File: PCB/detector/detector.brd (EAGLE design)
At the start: 53.3 x 51.7 mm, 36 parts, among them IC1 STM32F042K6T6

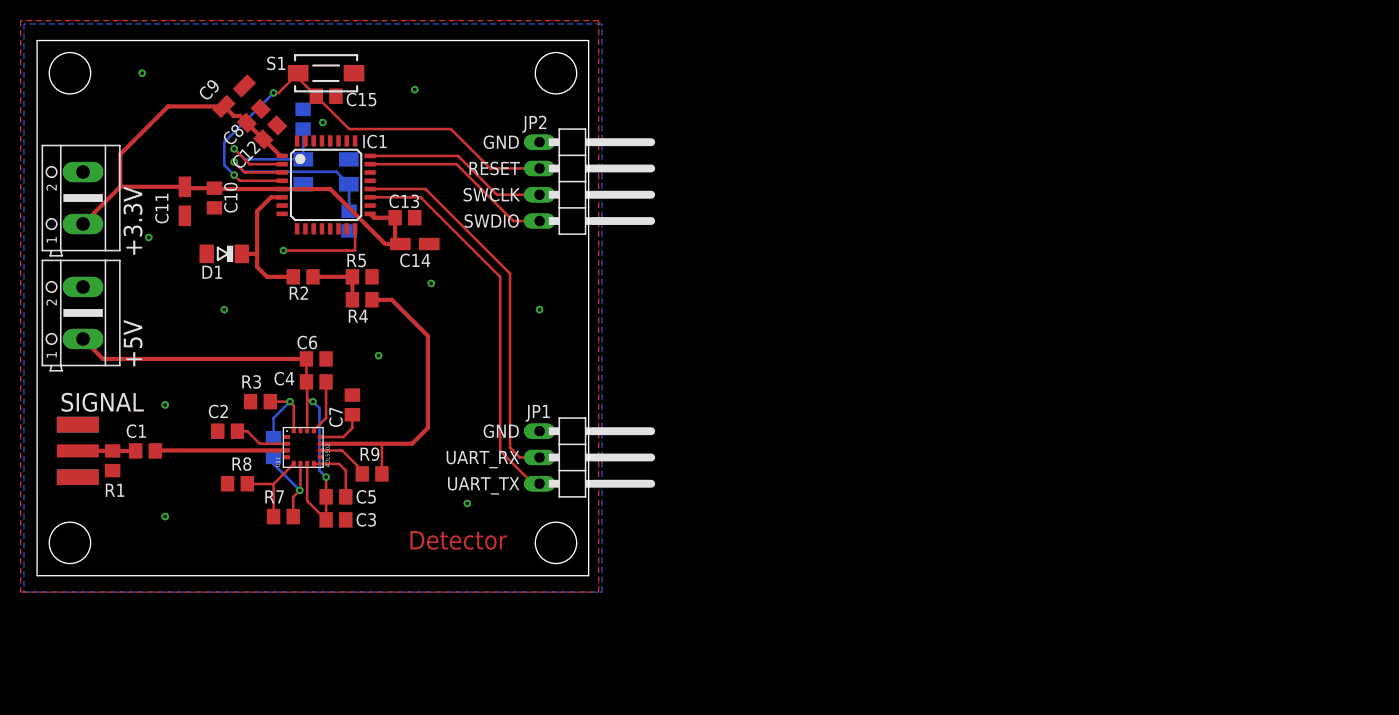
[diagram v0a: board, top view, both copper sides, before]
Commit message: almost ready
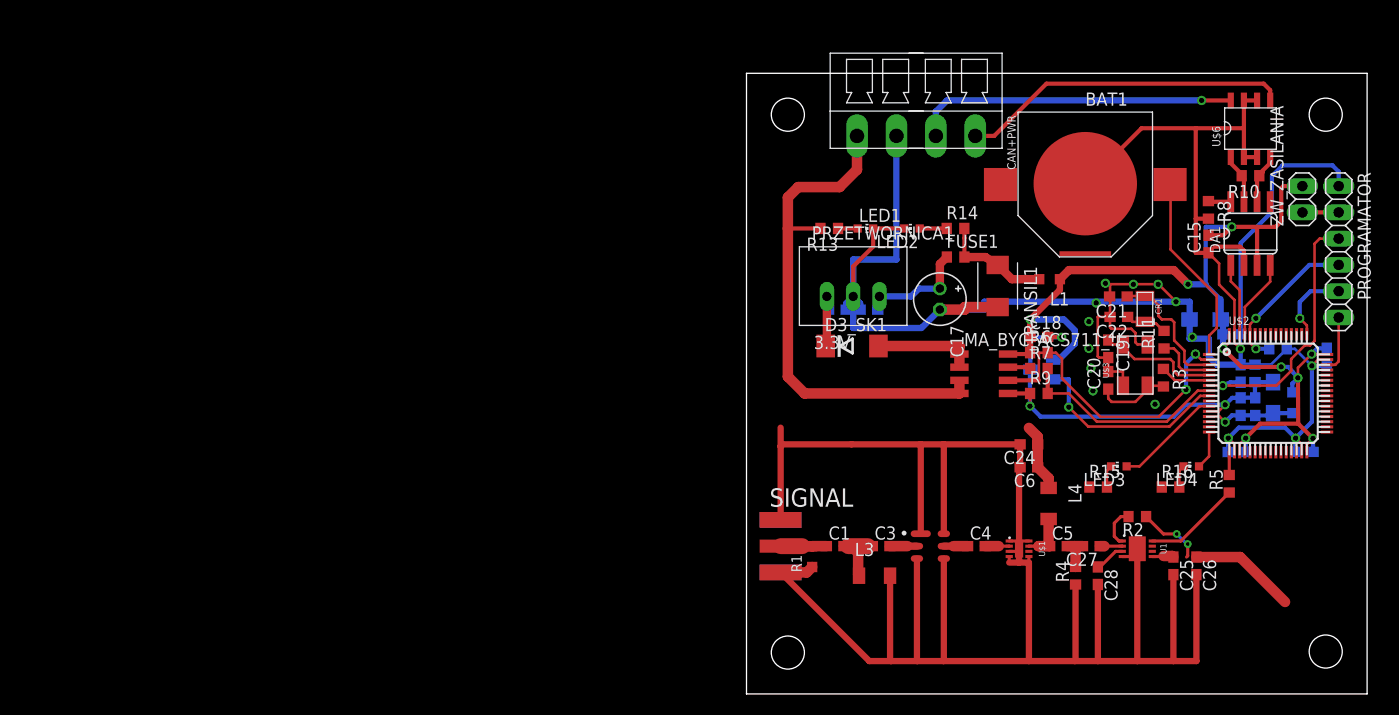
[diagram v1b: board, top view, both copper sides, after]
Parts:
- removed +3.3V, +5V: (no value), con-ptr500:AK500/2
- removed D1: 3.3V, diode:SOD80C
- removed JP1: (no value), pinhead:1X03/90
- removed JP2: (no value), pinhead:1X04/90
- removed Q1: (no value), crystal:CTS406
- removed S1: DTSM-3, swtich:DTSM-3
- added BAT1: BAT_3V, battery CR1216:CR1216
- added C18, C23: 100nF, resistor:C0603
- added C19, C20, C21, C22: 22pF, resistor:C0603
- added C24: 1u, rcl:C0603
- added C25: 100p, rcl:C0603
- added C26: 100n, rcl:C0603
- added C27, C28: 1n, rcl:C0603
- added CAN+PWR: 4PIN_3.81_KATOWA, zielone raster 3.81:CON-PHOENIX_3.81-4PIN_KAT
- added CR1: 32,768kHz, crystal_scorpio:IL3X
- added D3_SK1: 5A, diode:DO214AA
- added DA1: SN65HVD230, can_driver:SO08
- added FUSE1: 3A, resistor:R0603
- added L1: 1uH/500mA, rcl:L2012C
- added L2: 10uH/20mA, rcl:L2012C
- added L3, L4: (no value), rcl:L3216C
- added LED1, LED3: zielona, led:CHIP-LED0603
- added LED2: niebieska, led:CHIP-LED0603
- added LED4: czerwona, led:CHIP-LED0603
- added MA_BYC_ACS711_!!: ACS712, acs712:SO08
- added PROGRAMATOR: (no value), pinhead:1X06
- added PRZETWORNICA1: 3.3V, OKI-78SR:TO220
- added R10: 120R*, resistor:R0603
- added R11: 390k, resistor:R0603
- added R12, R13: 10k, resistor:R0603
- added R14, R15, R16: 470R, resistor:R0603
- added TRANSIL1: 3.3V, diode:SMBJ
- added U$2: STM32F072RBT6, STM32F072RBT6:TQFP64
- added U$3: ABM3, crystal_scorpio:ABM3
- added U$6: LC03-6R2G, LC03-6R2 - diody ESD do magistrali:SOIC-8
- added U1: LT5538, DFN-8:DFN-8_3X3
- added U2: B39431B3710U410, SON120P300X300X110-6N:SON120P300X300X110-6N
- added ZW_MASY: (no value), resistor:R0603
- added ZW_ZASILANIA: (no value), pinhead:1X02
- C1: value 100n -> (none); device rcl:C0805 -> rcl:C0603
- C10, C12, C15: value 100n -> 100nF; device rcl:C0805 -> resistor:C0603
- C11, C9: value 4.7u -> 100nF; device rcl:CT3216 -> resistor:C0603
- C13: value 10n -> 100nF; device rcl:C0805 -> resistor:C0603
- C14: value 1u -> 100nF; device rcl:CT3216 -> resistor:C0603
- C16: value 20p -> 100nF; device rcl:C0805 -> resistor:C0603
- C17: value 20p -> 6,3V/100uF; device rcl:C0805 -> resistor:E2-5
- C2: value 100p -> 4,7uF; device rcl:C0805 -> rcl:SMC_A
- C3: value 100p -> (none); device rcl:C0805 -> rcl:C0603
- C4: device rcl:C0805 -> rcl:C0603
- C5, C6: value 100n -> 100p; device rcl:C0805 -> rcl:C0603
- C7: value 10u -> 4,7uF; device rcl:C0805 -> rcl:SMC_A
- C8: value 100n -> 1uF; device rcl:C0805 -> resistor:C0603
- IC1: value STM32F042K6T6 -> LM50; device STM32F042K6T6:QFP80P900X900X160-32N -> linear:SOT23
- R1: value 60.4R -> VARISTORCN0603; device rcl:R0805 -> varistor:CT/CN0603
- R2: value 2k -> (none); device rcl:R0805 -> rcl:R0603
- R3: value 301R -> 820R; device rcl:R0805 -> resistor:R0603
- R4: value 10k -> 56R; device rcl:R0805 -> rcl:R0603
- R5: value 20k -> (none); device rcl:R0805 -> rcl:R0603
- R6: value 1430R -> 10k; device rcl:R0805 -> resistor:R0603
- R7: value 3.74k -> 100K; device rcl:R0805 -> resistor:R0603
- R8: value 2k -> ZW 0-100K; device rcl:R0805 -> resistor:R0603
- R9: value 0R -> 32k; device rcl:R0805 -> resistor:R0603
- U$1: value ADL5902 -> TQP3M9036; device ADL5902:ADL5902 -> DFN-8:DFN-8_2X2
- moved C11 111.4 mm to (127.2, 23.7), flipped to the bottom
- moved C9 101.8 mm to (118.9, 18.9), flipped to the bottom, turned to 90 degrees
- moved C8 100.8 mm to (120.3, 18.9), flipped to the bottom, turned to 90 degrees
- moved C10 99.2 mm to (118.0, 25.9), flipped to the bottom, turned to 180 degrees
- moved C12 98.4 mm to (118.5, 14.5), flipped to the bottom, turned to 0 degrees
- moved R8 97.5 mm to (115.8, 37.9), turned to 270 degrees
- moved C2 95.1 mm to (115.5, 27.3), flipped to the bottom, turned to 0 degrees
- moved C13 89.8 mm to (125.0, 14.5), flipped to the bottom
- moved C7 89.0 mm to (122.0, 19.8), flipped to the bottom
- moved R3 87.3 mm to (111.4, 21.7), turned to 270 degrees
- moved C15 86.5 mm to (115.8, 34.6), turned to 90 degrees
- moved R5 86.2 mm to (117.8, 11.4), turned to 90 degrees
- moved R2 83.9 mm to (108.9, 8.26), turned to 180 degrees
- moved R6 74.6 mm to (99.4, 24.1), flipped to the top, turned to 0 degrees
- moved R7 74.4 mm to (99.4, 22.6)
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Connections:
- net N$1 renamed SIGNAL
- removed net +5V: +5V.1, C3.1, C4.1, C5.1, C6.1, U$1.P$10, U$1.P$3
- removed net ADC_IN: D1.C, IC1.6, R2.1
- removed net INHI: C1.2, U$1.P$14
- removed net OSC_IN: C17.1, IC1.2, Q1.3
- removed net OSC_OUT: C16.1, IC1.3, Q1.1
- removed net RESET: C15.1, IC1.4, JP2.2, S1.1
- removed net SWCLK: IC1.24, JP2.3
- removed net UART_RX: IC1.20, JP1.2
- removed net UART_TX: IC1.19, JP1.3
- removed net VOUT: R4.2, R9.2, U$1.P$6
- new net +24V: C14.1, D3_SK1.C, PRZETWORNICA1.P1
- new net AGND: C18.2, C7.-, C8.2, C9.2, IC1.3, MA_BYC_ACS711_!!.5, R9.1, U$2.12, ZW_MASY.2
- new net AMP_OUT: C27.2, C5.2, R4.2
- new net BOOT_0: PROGRAMATOR.4, R12.2, U$2.60
- new net CANH_1: DA1.7, R10.2, U$6.1
- new net CANL_1: DA1.6, R10.1, U$6.4
- new net CAN_RX_1: DA1.4, U$2.61
- new net CAN_TX_1: DA1.1, U$2.62
- new net DET_OUT: R5.2, U$2.17
- new net FILTER_IN: C3.2, U2.2
- new net FILTER_OUT: C4.1, U2.5
- new net LED1: LED3.A, U$2.11
- new net LED2: LED4.A, U$2.16
- new net N$1: MA_BYC_ACS711_!!.7, R7.1
- new net N$10: C19.1, U$2.5, U$3.P$2
- new net N$11: C4.2, U$1.2
- new net N$12: CAN+PWR.P$2, U$6.8
- new net N$13: R11.1, U$2.4
- new net N$14: C21.1, CR1.P$1, U$2.3
- new net N$15: C22.1, CR1.P$2, R11.2
- new net N$16: CAN+PWR.P$1, U$6.5
- new net N$18: LED1.A, R13.1
- new net N$19: LED2.A, R14.1
- new net N$20: LED3.C, R15.2
- new net N$21: LED4.C, R16.2
- new net N$22: C28.1, U1.3
- new net N$23: C27.1, U1.2
- new net N$24: PROGRAMATOR.2, ZW_ZASILANIA.1
- new net N$25: R2.2, U1.1
- new net N$27: C5.1, L4.2, U$1.7
- new net N$28: U1.7
- new net N$29: U1.6
- new net N$8: D3_SK1.A, MA_BYC_ACS711_!!.1, MA_BYC_ACS711_!!.2
- new net NRST: C23.1, PROGRAMATOR.3, U$2.7
- new net OVER_CURRENT: MA_BYC_ACS711_!!.6, R6.2, U$2.2
- new net PRAD_PLYTKI: R7.2, R9.2, U$2.8
- new net SWD_CLK: PROGRAMATOR.5, U$2.49
- new net TEMP: IC1.2, U$2.9
- new net VBAT: BAT1.P$1, BAT1.P$2, BAT1.P$3, U$2.1
- new net VCC: CAN+PWR.P$4, MA_BYC_ACS711_!!.3, MA_BYC_ACS711_!!.4, R13.2
- new net VDD: C10.1, C11.1, C12.1, C13.1, C15.2, C18.1, C2.+, DA1.3, IC1.1, L1.1, L2.1, MA_BYC_ACS711_!!.8, R6.1, U$2.19, U$2.32, U$2.48, U$2.64, ZW_ZASILANIA.2
- net +3V3: now also C24.1, C25.1, C26.1, C6.1, FUSE1.2, L1.2, L4.1, R14.2, R2.1, TRANSIL1.C, U1.5; no longer +3.3V.1, C10.1, C11.+, C12.1, C13.1, C14.+, C8.1, C9.+, IC1.1, IC1.17, IC1.5
- net GND: now also BAT1.P$4, C11.2, C14.2, C15.1, C17.-, C19.2, C2.-, C20.2, C21.2, C22.2, C23.2, C24.2, C25.2, C26.2, C28.2, CAN+PWR.P$3, DA1.2, L3.2, LED1.C, LED2.C, PROGRAMATOR.1, PRZETWORNICA1.P2, R12.1, R15.1, R16.1, R4.1, R8.2, TRANSIL1.A, U$1.1, U$1.3, U$1.4, U$1.5, U$1.8, U$1.PAD, U$2.18, U$2.31, U$2.47, U$2.63, U$3.P$1, U$3.P$3, U$6.2, U$6.3, U$6.6, U$6.7, U1.4, U1.9, U2.1, U2.3, U2.4, U2.6, ZW_MASY.1; no longer +3.3V.2, +5V.2, C11.-, C14.-, C15.2, C17.2, C2.2, C3.2, C4.2, C5.2, C7.2, C8.2, C9.-, D1.A, IC1.16, IC1.32, JP1.1, JP2.1, R3.1, R5.1, R8.1, S1.2, U$1.P$4, U$1.P$9
- net N$2: now also C16.1, C17.+, FUSE1.1, PRZETWORNICA1.P3; no longer R6.2, R7.2, U$1.P$11
- net N$3: now also R3.1, U$2.6; no longer C2.1, U$1.P$15
- net N$4: now also C7.+, C8.1, C9.1, L2.2, U$2.13; no longer C7.1, U$1.P$5
- net N$5: now also C1.2, C3.1, L3.1; no longer R2.2, R4.1, R5.2
- net N$6: now also C20.1, R3.2, U$3.P$4; no longer R9.1, U$1.P$7
- net N$7: now also DA1.8, R8.1; no longer R3.2, R6.1, U$1.P$1
- net N$9: now also R5.1, U1.8; no longer R7.1, R8.2, U$1.P$12
- net SWDIO: now also PROGRAMATOR.6, U$2.46; no longer IC1.23, JP2.4
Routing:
- net GND: track 20.1 -> 423.6 mm, vias 12 -> 15
- net VDD: track 0.00 -> 101.9 mm, vias 0 -> 9
- net VCC: track 0.00 -> 50.3 mm
- net +5V: track 48.1 -> 0.00 mm, vias 2 -> 0
- net RESET: track 45.8 -> 0.00 mm, vias 2 -> 0
- net AGND: track 0.00 -> 42.5 mm, vias 0 -> 3
- net UART_TX: track 37.7 -> 0.00 mm
- net UART_RX: track 37.0 -> 0.00 mm
- net N$16: track 0.00 -> 31.9 mm
- net N$12: track 0.00 -> 31.3 mm, vias 0 -> 1
- net OVER_CURRENT: track 0.00 -> 30.0 mm, vias 0 -> 2
- net VOUT: track 29.7 -> 0.00 mm
- net +3V3: track 62.7 -> 36.3 mm, vias 0 -> 2
- net NRST: track 0.00 -> 26.4 mm, vias 0 -> 1
- net PRAD_PLYTKI: track 0.00 -> 20.4 mm
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- removed copper zone on layer 1, net GND
- removed copper zone on layer 16, net GND
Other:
- board size 53.3 x 51.7 mm -> 60 x 60 mm
- board text removed: "Detector"
- board text removed: "GND"
- board text removed: "RESET"
- board text removed: "SWCLK"
- board text removed: "SWDIO"
- board text removed: "UART_RX"
- board text removed: "UART_TX"
